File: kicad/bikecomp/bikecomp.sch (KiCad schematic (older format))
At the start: 8 parts

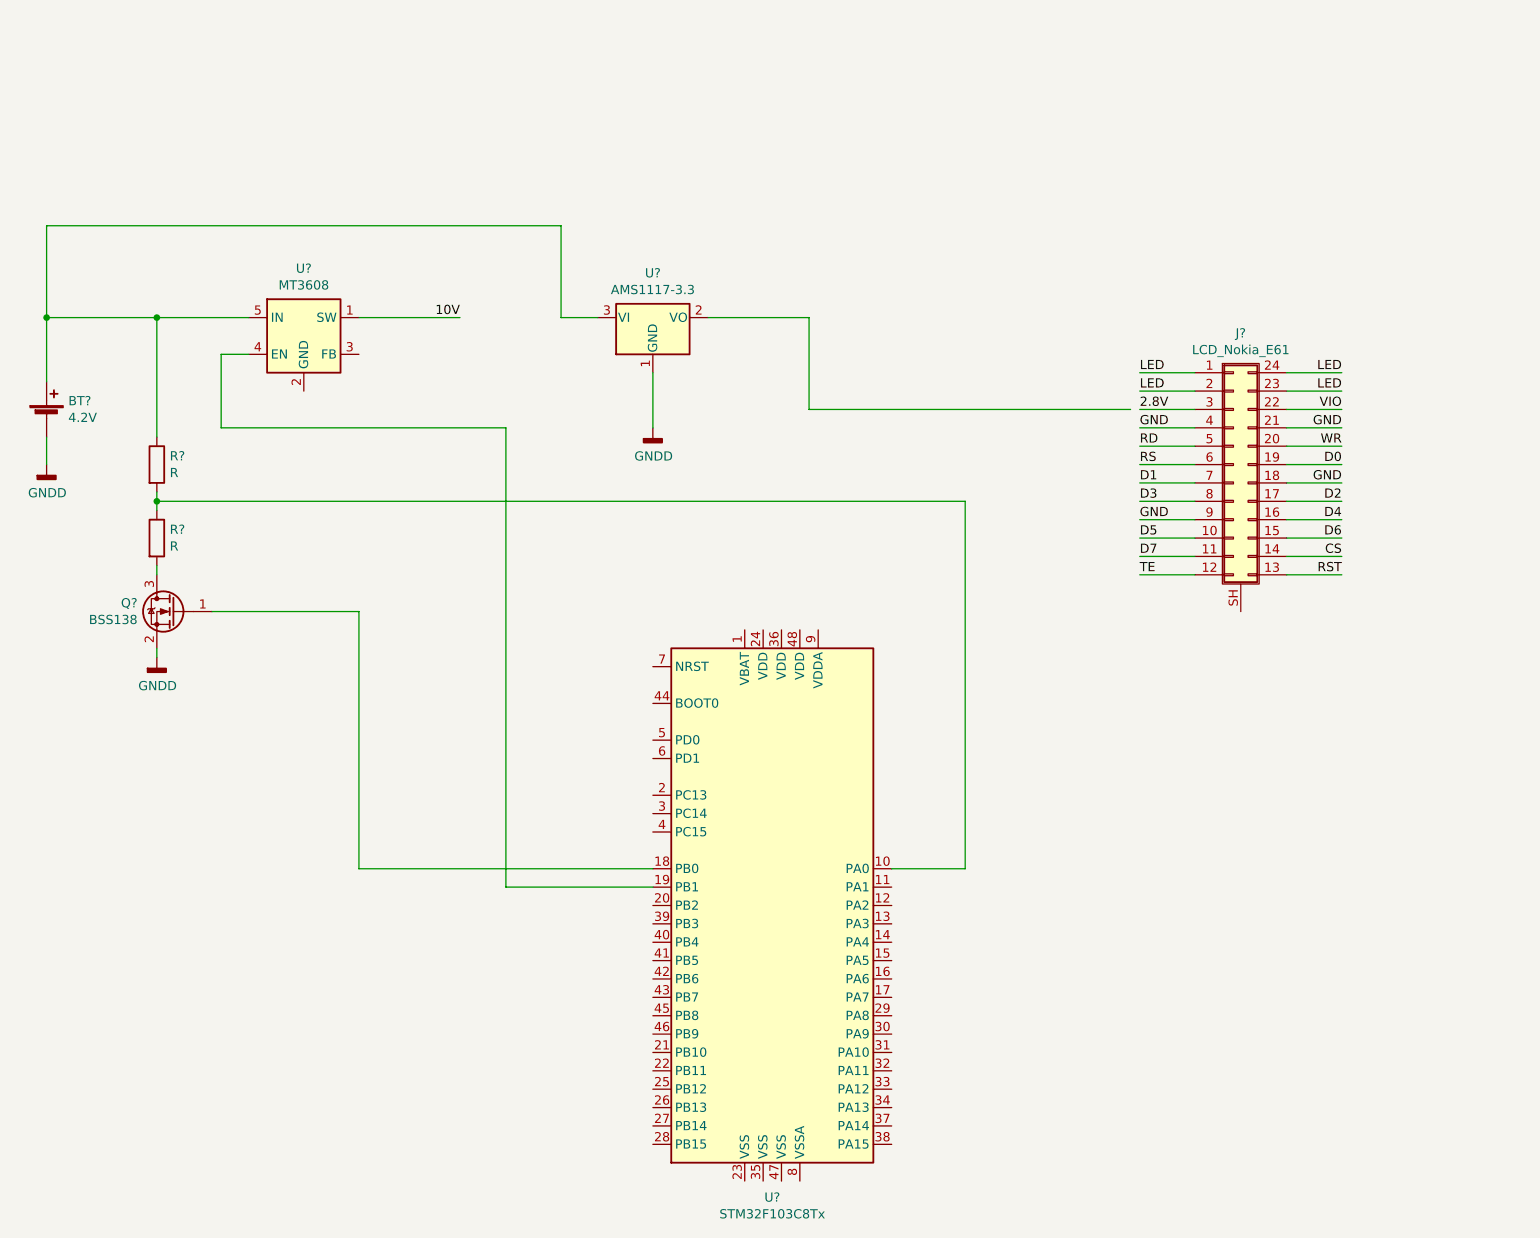
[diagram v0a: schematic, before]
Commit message: Schematics experiments
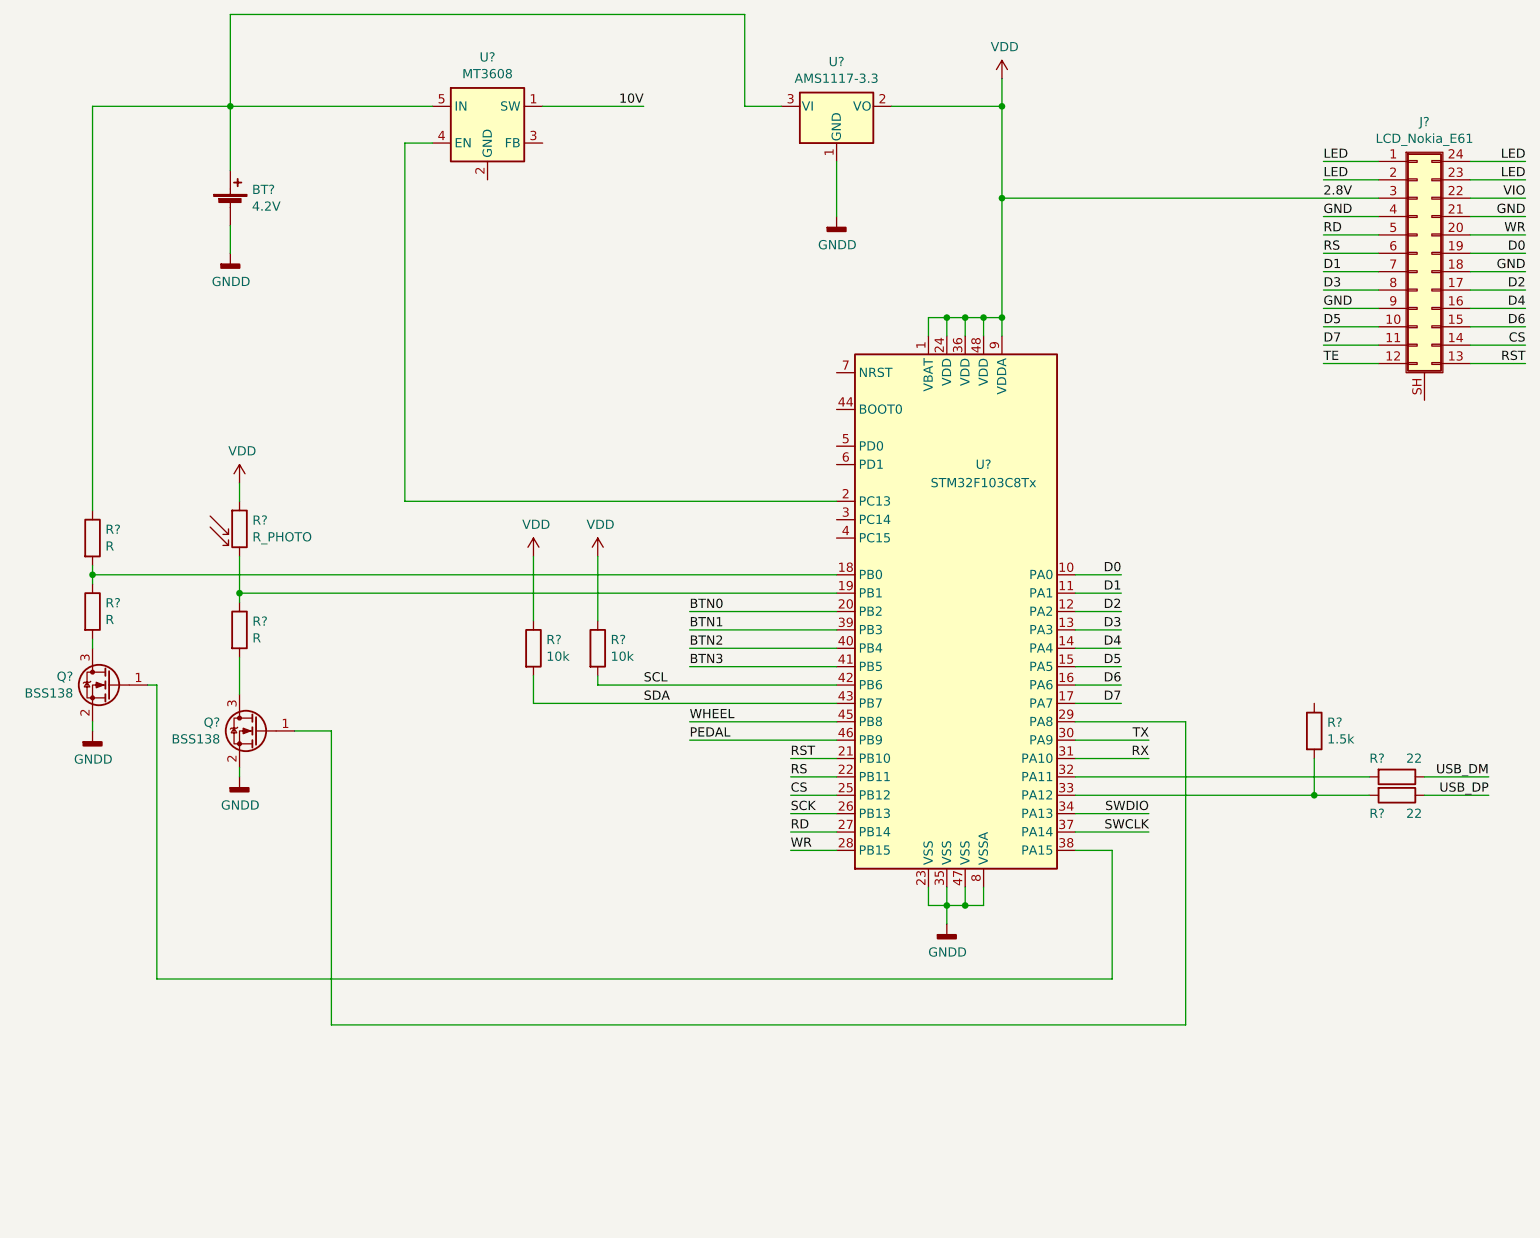
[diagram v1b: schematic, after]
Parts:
- added Q?: BSS138, Package_TO_SOT_SMD:SOT-23, symbol Transistor_FET:BSS138
- added R? (x2): 22, symbol Device:R
- added R?: 1.5k, symbol Device:R
- added R? (x2): 10k, symbol Device:R
- added R?: R, symbol Device:R
- added R?: R_PHOTO, symbol Device:R_PHOTO
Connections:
- net 2.8V is gone; now on net VDD: J?.3 (Pin_3)
- net CS: now also U?.25 (PB12)
- net D0: now also U?.10 (PA0)
- net D1: now also U?.11 (PA1)
- net D2: now also U?.12 (PA2)
- net D3: now also U?.13 (PA3)
- net D4: now also U?.14 (PA4)
- net D5: now also U?.15 (PA5)
- net D6: now also U?.16 (PA6)
- net D7: now also U?.17 (PA7)
- net GNDD: now also U?.23 (VSS), U?.35 (VSS), U?.47 (VSS), U?.8 (VSSA), Q?.2 (S)
- net RD: now also U?.27 (PB14)
- net RS: now also U?.22 (PB11)
- net RST: now also U?.21 (PB10)
- net WR: now also U?.28 (PB15)
- net VDD: now reaches U?.2 (VO)
- net VDD: now also U?.1 (VBAT), U?.24 (VDD), U?.36 (VDD), U?.48 (VDD), U?.9 (VDDA), R?.1, R?.1, R?.1
- net at U?.4 (EN): now also U?.2 (PC13); no longer U?.19 (PB1)
- net at R?.1, R?.2: now also U?.18 (PB0); no longer U?.10 (PA0)
- net at Q?.1 (G): now also U?.38 (PA15); no longer U?.18 (PB0)
- net BTN0: now reaches U?.20 (PB2)
- net SCK: now reaches U?.26 (PB13)
- net at U?.29 (PA8): now also Q?.1 (G)
- net TX: now reaches U?.30 (PA9)
- net RX: now reaches U?.31 (PA10)
- net at U?.32 (PA11): now also R?.2
- net at U?.33 (PA12): now also R?.2, R?.2
- net SWDIO: now reaches U?.34 (PA13)
- net SWCLK: now reaches U?.37 (PA14)
- net BTN1: now reaches U?.39 (PB3)
- net BTN2: now reaches U?.40 (PB4)
- net BTN3: now reaches U?.41 (PB5)
- net SCL: now reaches U?.42 (PB6)
- net SCL: now also R?.2
- net SDA: now reaches U?.43 (PB7)
- net SDA: now also R?.2
- net WHEEL: now reaches U?.45 (PB8)
- net PEDAL: now reaches U?.46 (PB9)
- new net: R?.1, R?.2, U?.19 (PB1)
- new net: Q?.3 (D), R?.2
- new net USB_DM: R?.1
- new net USB_DP: R?.1
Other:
- moved on the sheet: BT?, J?, Q?, R?, U?
